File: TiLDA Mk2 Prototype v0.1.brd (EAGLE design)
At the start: 67.9 x 100 mm, 200 parts, among them IC1 ATSAM3X8EA-AU, IC10 MCP73831, IC2 MPU-6050, IC3 SRF-V1.2, IC5 S25FL216K0PMFI011, IC7 HMC5883LSMD (NP), IC8 MCP1825T-3302E/DC, IC9 TC1015-3V3, J1 ZX62-AB-5PA(11), J3 Arduino Headers, J5 1050270001 (NP), J6 B016 - PowerPOD NCP1402 5V0, J7 SFV30R-2STE1HLF, J8 1x02 RA Pin, Q10 2N7002KW, Q11 BSS84W, Q12 2N7002KW, Q13 BSS84W, Q14 NTR1P02T1G, Q8 BSS84W, Q9 2N7002KW, U2 JHD12864-G13BSW-OUTLINE, X1 12Mhz 13pF 30ppm (7pf caps), X2 32.768Khz

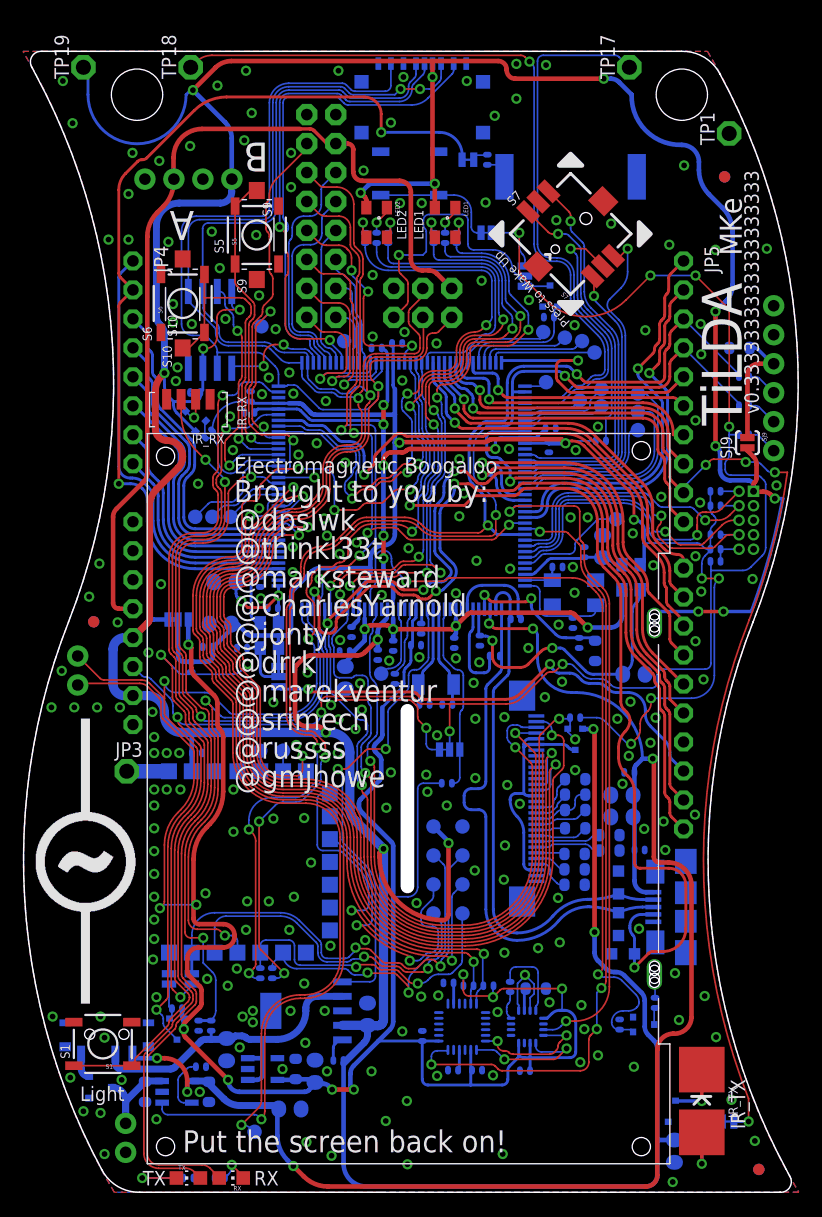
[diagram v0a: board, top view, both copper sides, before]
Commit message: Prototype: Minor schematic tweaks, board tweaks
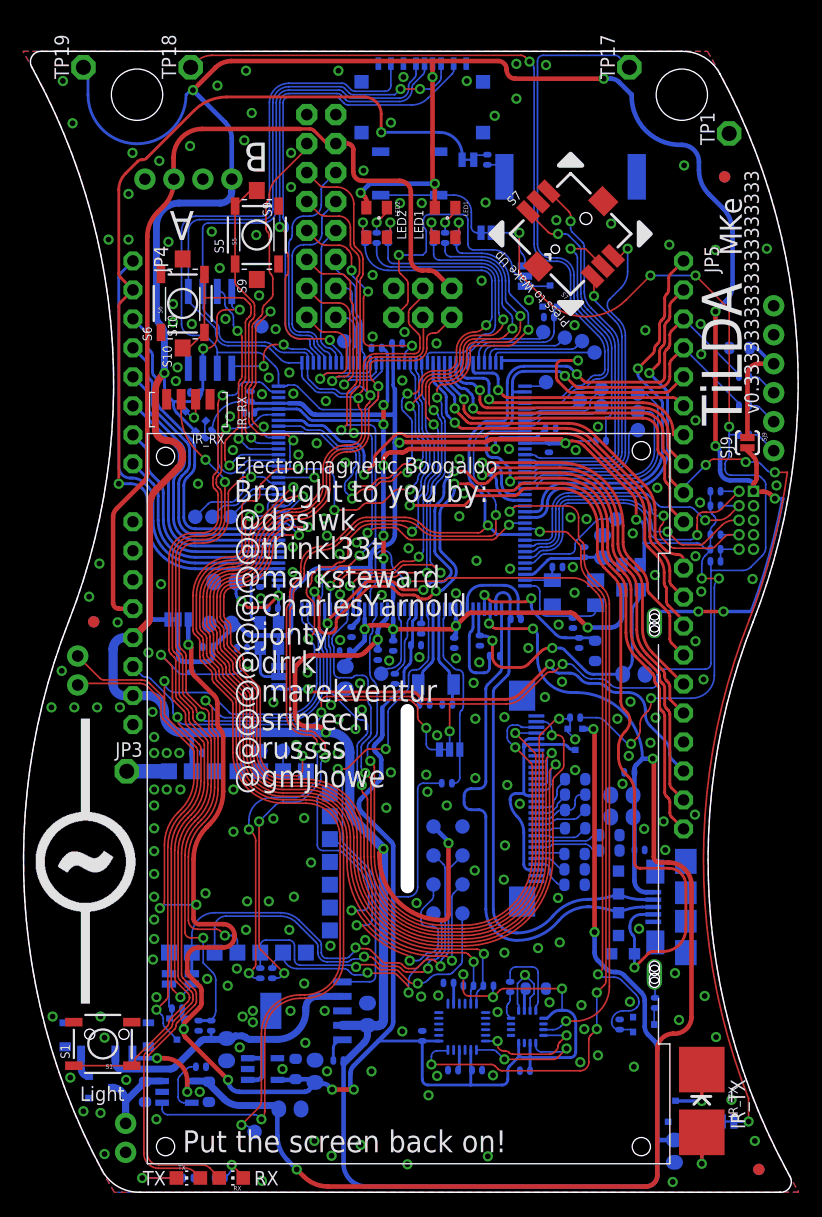
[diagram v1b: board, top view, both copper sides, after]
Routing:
- net GND: vias 239 -> 241
